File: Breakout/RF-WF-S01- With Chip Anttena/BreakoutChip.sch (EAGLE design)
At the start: 61 parts, among them U2 FT2232D, U3 LMR10510XMFE, U5 93LC46BT-I/OT

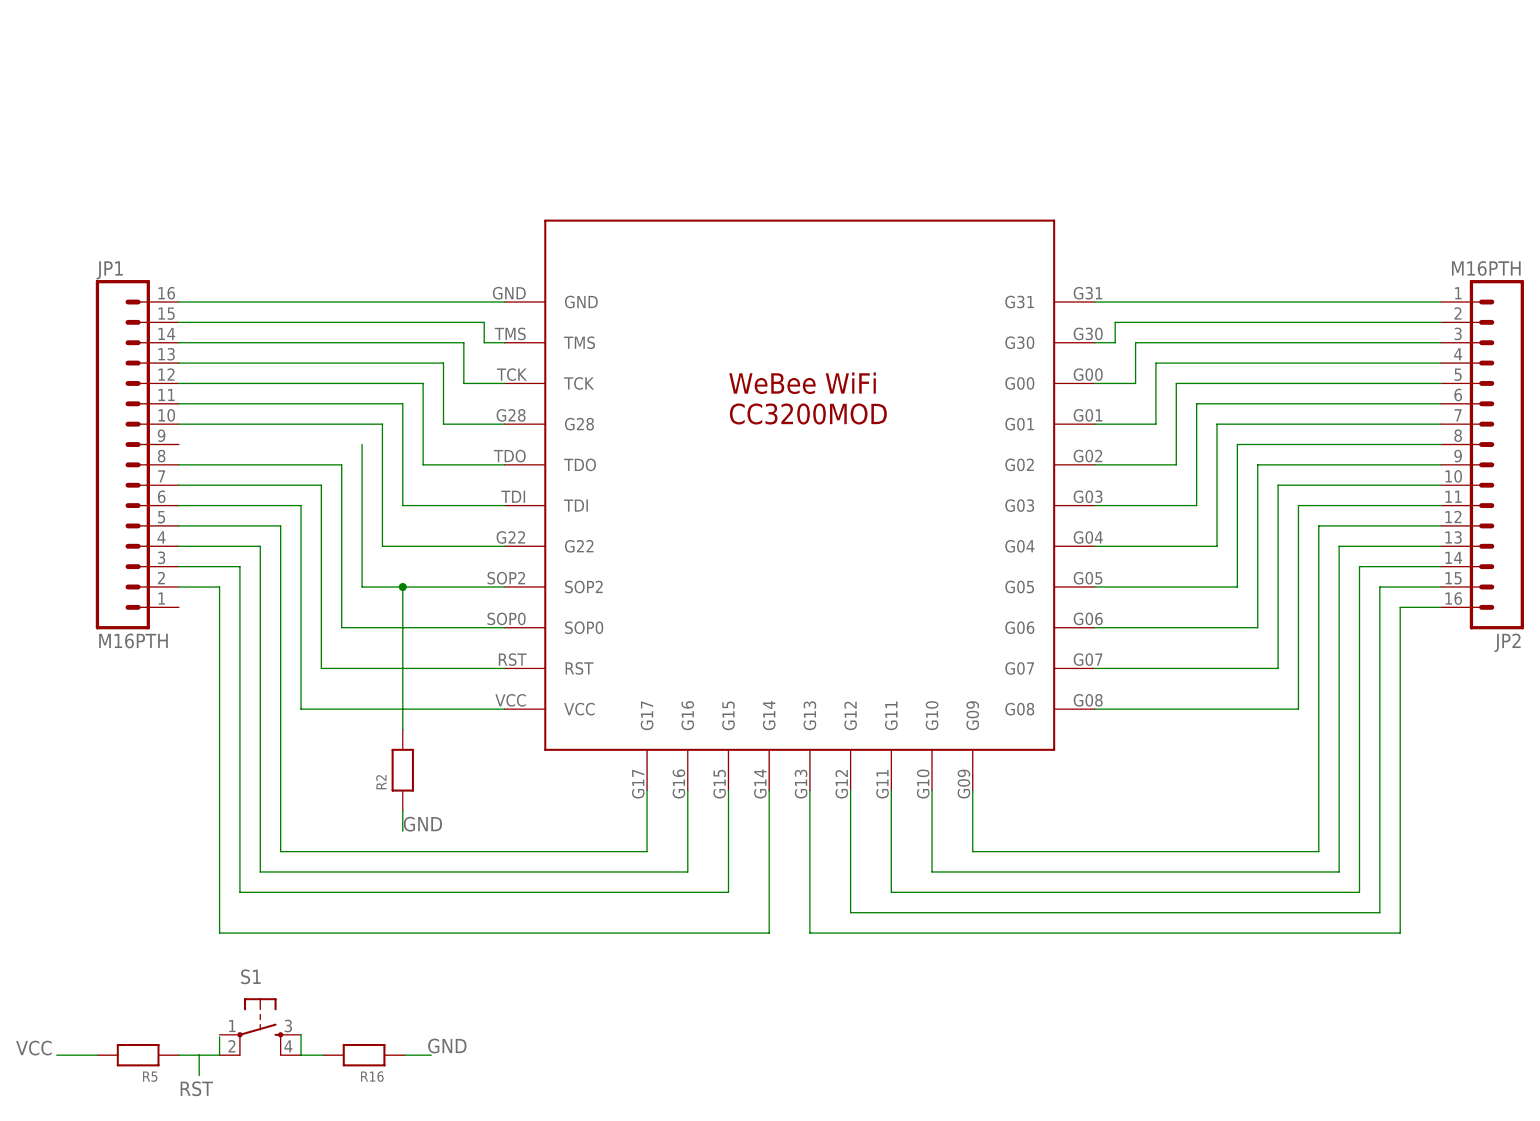
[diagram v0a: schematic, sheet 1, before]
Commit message: Some cleanup
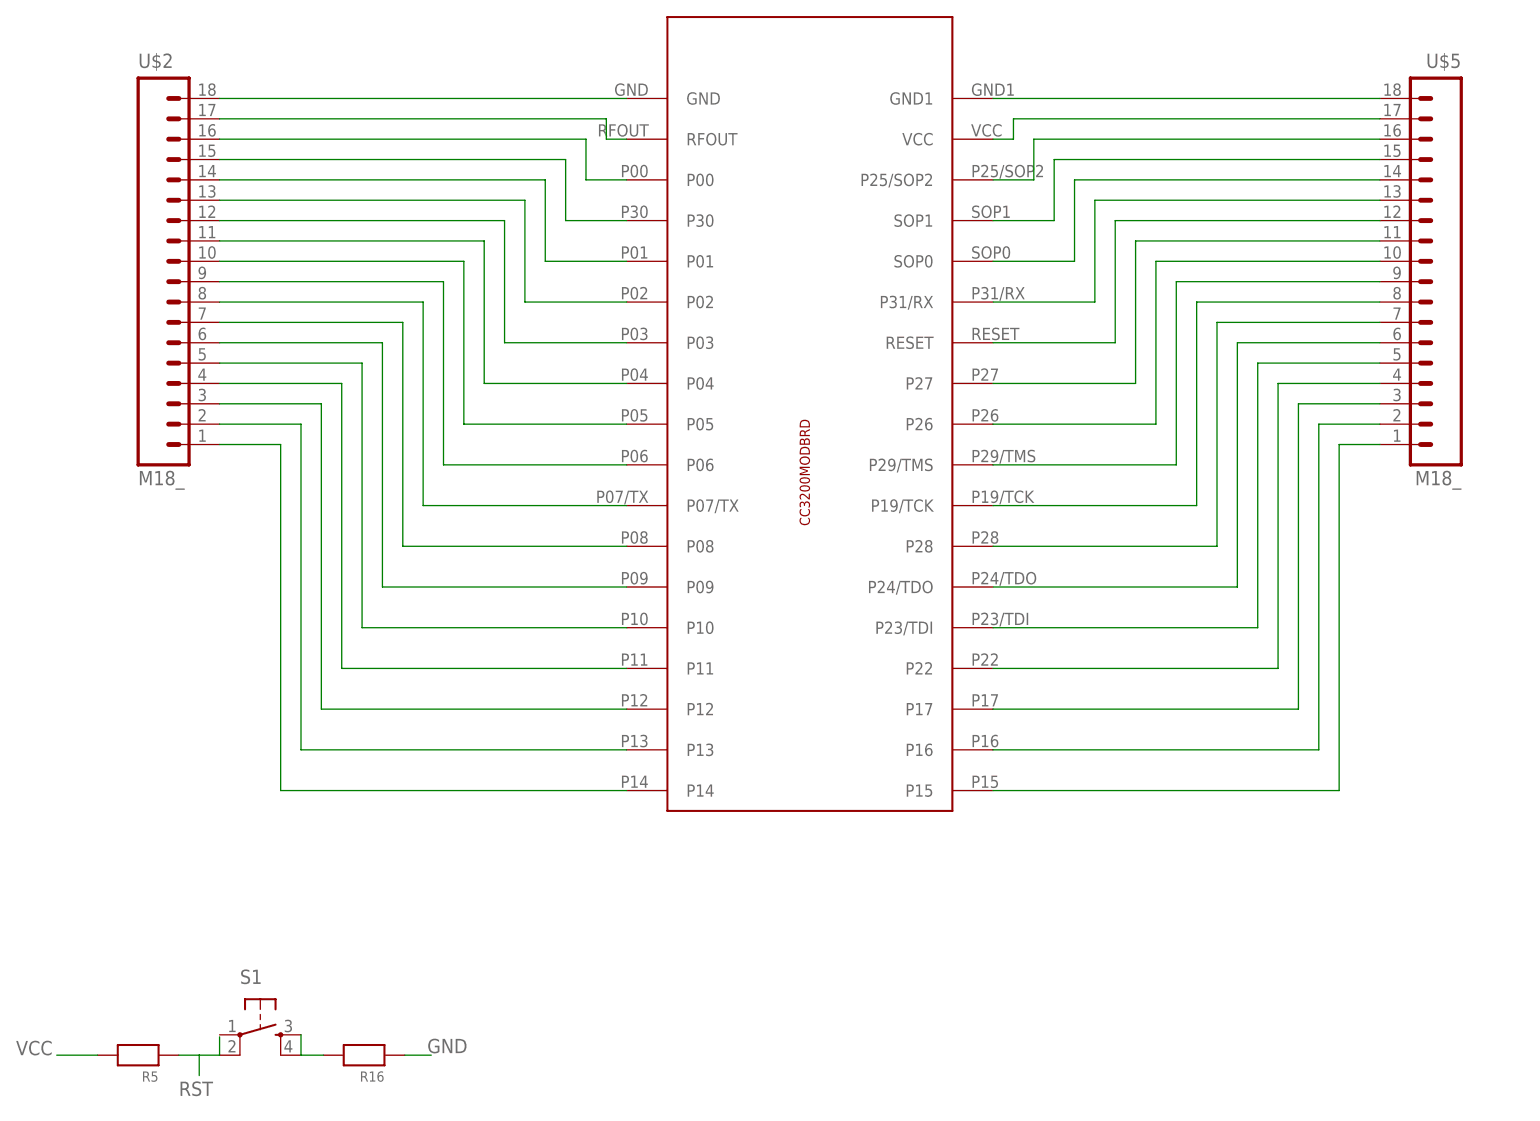
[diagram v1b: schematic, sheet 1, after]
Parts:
- removed JP1, JP2: M16PTH, DECADE-libraries:M16PTH
- removed R2: (no value), microbuilder:RESISTOR0402
- added U$2, U$5: M18_, DECADE-libraries:M18_
- U$1: value WEBEE_WIFI_CC3200 -> CC3200MOD; device WeeBee:WEBEE_WIFI_CC3200 -> CC3200MODBRD:CC3200MOD
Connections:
- removed net G00: JP2.3, U$1.G00
- removed net N$12: JP2.1, U$1.G31
- removed net N$2: JP1.15, U$1.TMS
- removed net N$22: JP2.11, U$1.G08
- removed net N$23: JP2.12, U$1.G09
- removed net N$24: JP1.5, U$1.G17
- removed net N$28: JP2.16, U$1.G13
- removed net N$6: JP1.11, U$1.TDI
- removed net N$7: JP1.10, U$1.G22
- new net N$10: U$1.P04, U$2.11
- new net N$14: U$1.P07/TX, U$2.8
- new net N$15: U$1.P08, U$2.7
- new net N$16: U$1.P09, U$2.6
- new net N$32: U$1.P19/TCK, U$5.8
- new net N$33: U$1.P28, U$5.7
- new net N$34: U$1.P24/TDO, U$5.6
- new net N$35: U$1.P23/TDI, U$5.5
- new net N$36: U$1.P22, U$5.4
- new net N$37: U$1.P17, U$5.3
- new net N$52: U$1.P16, U$5.2
- new net N$53: U$1.P15, U$5.1
- net FTDI_RX: now also U$1.P01, U$2.14; no longer JP2.4, U$1.G01
- net FTDI_TX: now also U$1.P02, U$2.13; no longer JP2.5, U$1.G02
- net GND: now also U$1.GND1, U$2.18, U$5.18; no longer JP1.16, R2.1
- net GPIO_05: now also U$1.P05, U$2.10
- net N$13: now also U$1.P06, U$2.9; no longer JP2.2, U$1.G30
- net N$17: now also U$1.P10, U$2.5; no longer JP2.6, U$1.G03
- net N$18: now also U$1.P11, U$2.4; no longer JP2.7, U$1.G04
- net N$19: now also U$1.P12, U$2.3; no longer JP2.8, U$1.G05
- net N$20: now also U$1.P13, U$2.2; no longer JP2.9, U$1.G06
- net N$21: now also U$1.P14, U$2.1; no longer JP2.10, U$1.G07
- net N$25: now also U$1.SOP1, U$5.15; no longer JP2.13, U$1.G10
- net N$26: now also U$1.SOP0, U$5.14; no longer JP2.14, U$1.G11
- net N$27: now also U$1.P31/RX, U$5.13; no longer JP2.15, U$1.G12
- net N$29: now also U$1.P27, U$5.11; no longer JP1.4, U$1.G16
- net N$3: now also U$1.RFOUT, U$2.17; no longer JP1.14, U$1.TCK
- net N$30: now also U$1.P26, U$5.10; no longer JP1.3, U$1.G15
- net N$31: now also U$1.P29/TMS, U$5.9; no longer JP1.2, U$1.G14
- net N$4: now also U$1.P00, U$2.16; no longer JP1.13, U$1.G28
- net N$5: now also U$1.P30, U$2.15; no longer JP1.12, U$1.TDO
- net N$9: now also U$1.P03, U$2.12; no longer JP1.8, U$1.SOP0
- net RST: now also U$1.RESET, U$5.12; no longer JP1.7, U$1.RST
- net SOP2: now also U$1.P25/SOP2, U$5.16; no longer R2.2, U$1.SOP2
- net VCC: now also U$5.17; no longer JP1.6
